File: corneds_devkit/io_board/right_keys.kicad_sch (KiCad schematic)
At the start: 42 parts, among them SW14 SW_Push, SW16 SW_Push, SW18 SW_Push, SW25 SW_Push, SW26 SW_Push, SW27 SW_Push, SW28 SW_Push, SW29 SW_Push, SW30 SW_Push, SW31 SW_Push, SW32 SW_Push, SW33 SW_Push, SW34 SW_Push, SW35 SW_Push, SW36 SW_Push, SW37 SW_Push, SW38 SW_Push, SW39 SW_Push, SW40 SW_Push, SW41 SW_Push, SW42 SW_Push

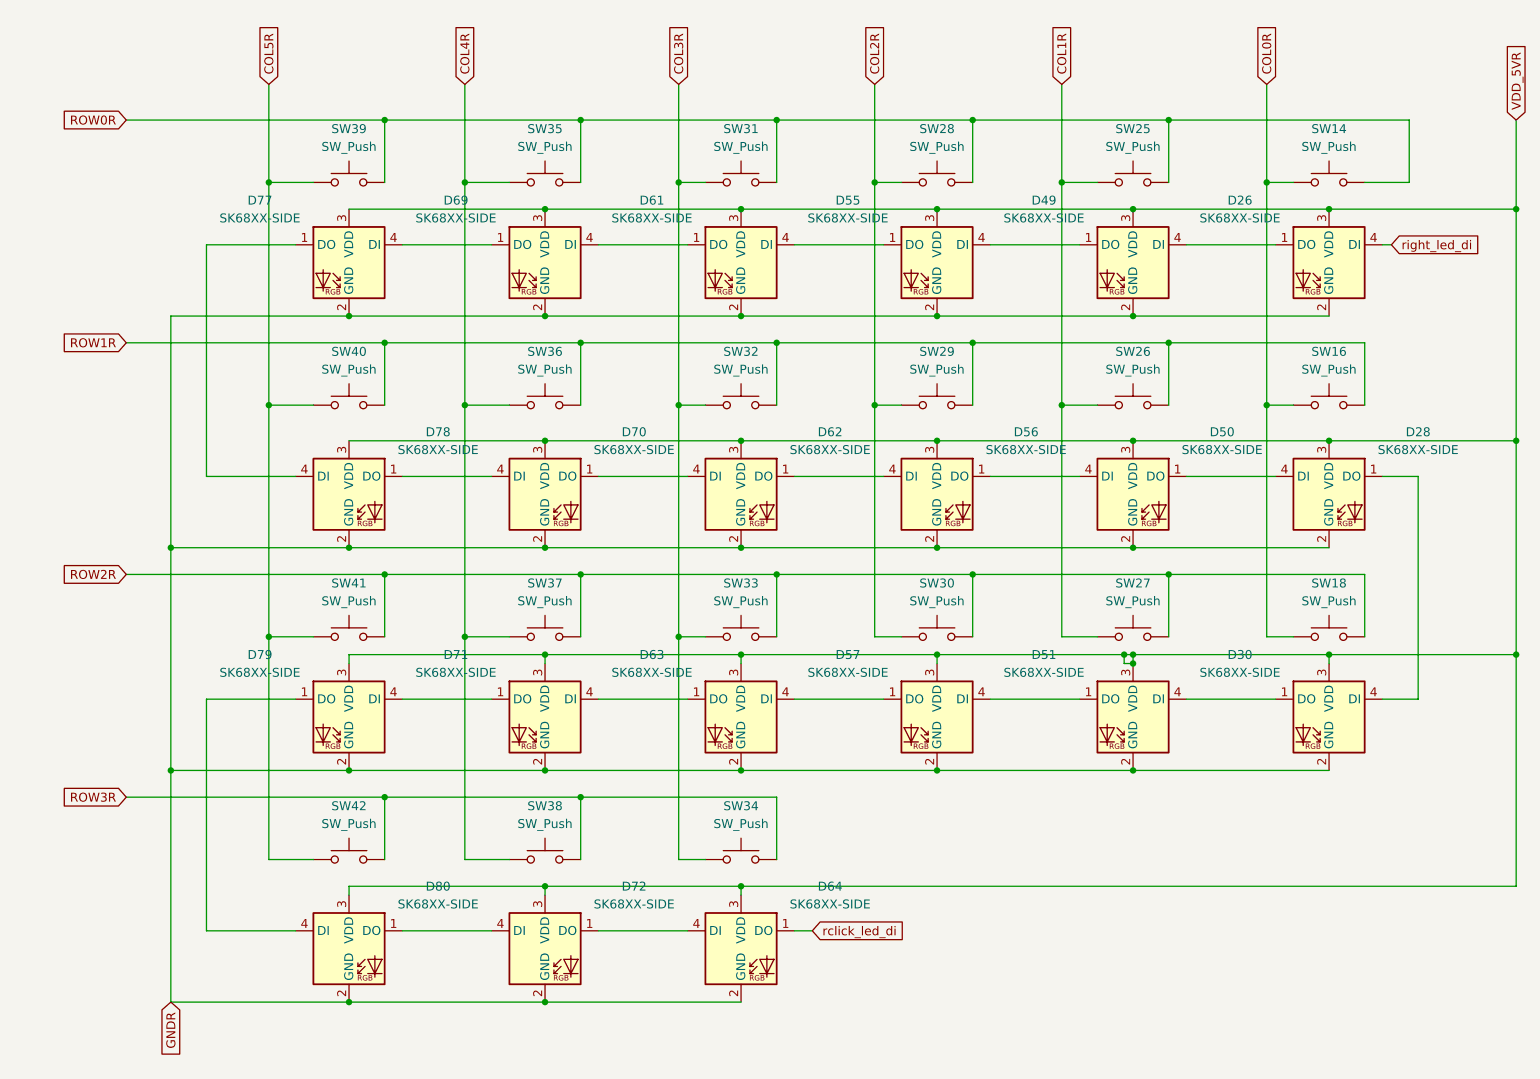
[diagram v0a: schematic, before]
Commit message: finished io board
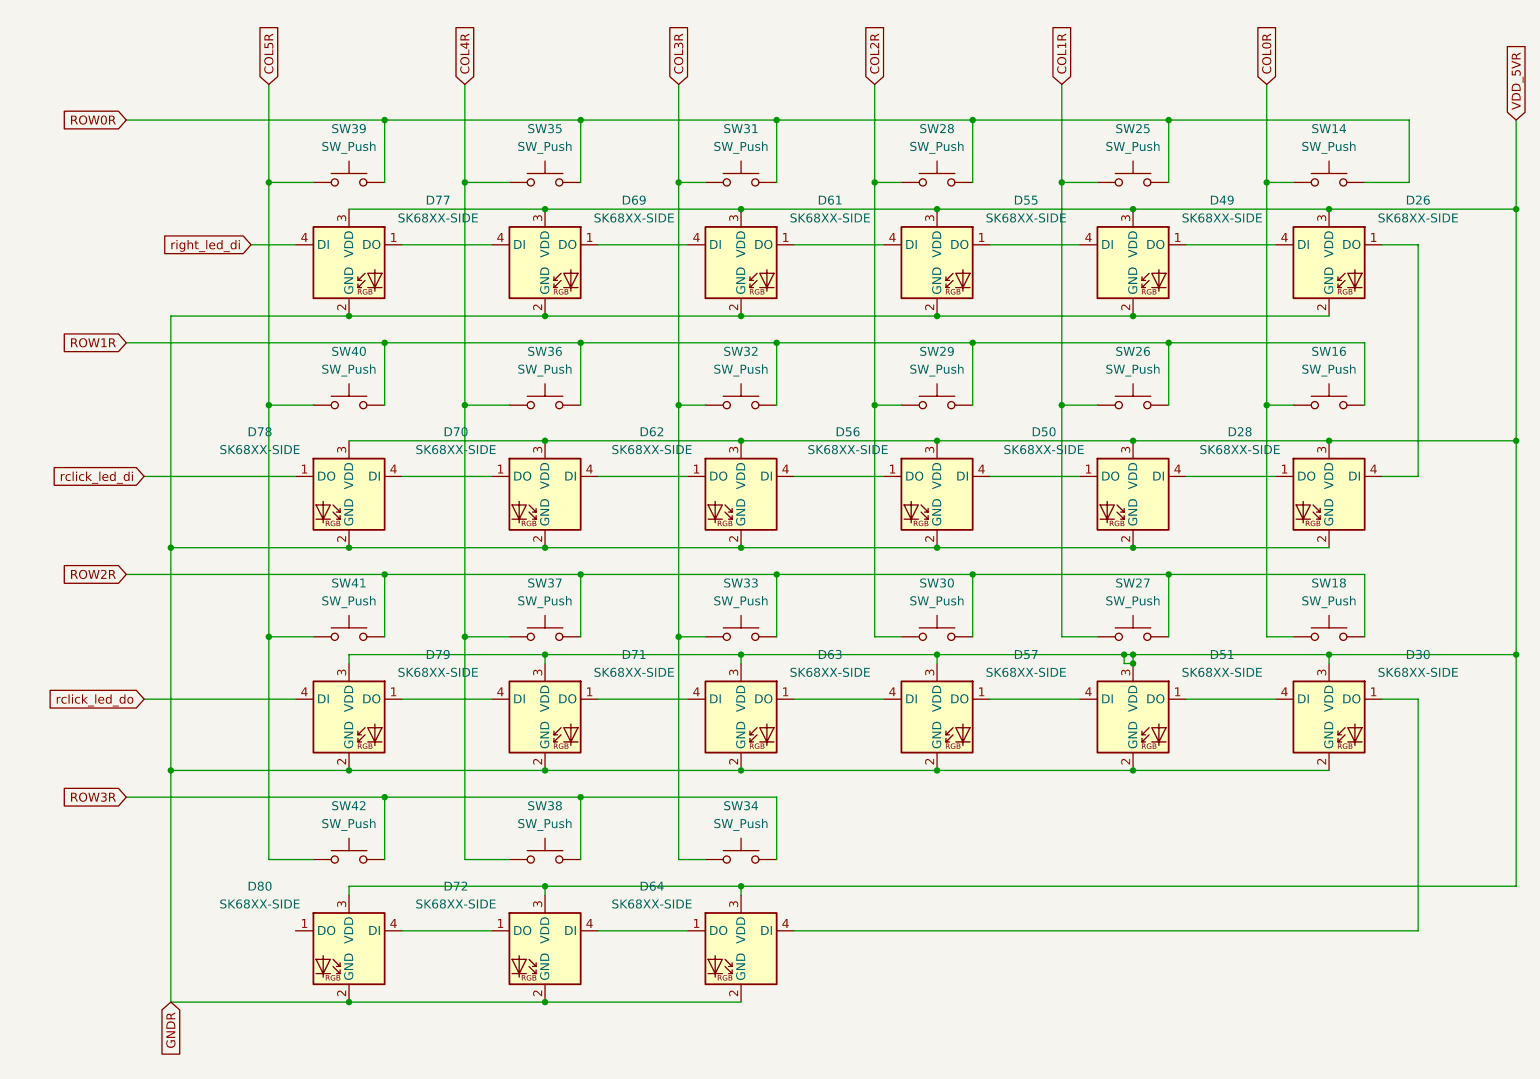
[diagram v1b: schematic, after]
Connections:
- net rclick_led_di: now also D78.1 (DO); no longer D64.1 (DO)
- net right_led_di: now also D77.4 (DI); no longer D26.4 (DI)
- net at D79.1 (DO): now also D71.4 (DI); no longer D80.4 (DI)
- net at D71.1 (DO): now also D63.4 (DI); no longer D79.4 (DI)
- net at D72.1 (DO): now also D80.4 (DI); no longer D64.4 (DI)
- net at D72.4 (DI): now also D64.1 (DO); no longer D80.1 (DO)
- net at D50.1 (DO): now also D56.4 (DI); no longer D28.4 (DI)
- net at D50.4 (DI): now also D28.1 (DO); no longer D56.1 (DO)
- net at D30.4 (DI): now also D51.1 (DO); no longer D28.1 (DO)
- net at D63.1 (DO): now also D57.4 (DI); no longer D71.4 (DI)
- net at D57.1 (DO): now also D51.4 (DI); no longer D63.4 (DI)
- net at D70.4 (DI): now also D62.1 (DO); no longer D78.1 (DO)
- net at D78.4 (DI): now also D70.1 (DO); no longer D77.1 (DO)
- net at D61.1 (DO): now also D55.4 (DI); no longer D69.4 (DI)
- net at D61.4 (DI): now also D69.1 (DO); no longer D55.1 (DO)
- net at D49.1 (DO): now also D26.4 (DI); no longer D55.4 (DI)
- net at D26.1 (DO): now also D28.4 (DI); no longer D49.4 (DI)
- net at D30.1 (DO): now also D64.4 (DI); no longer D51.4 (DI)
- net at D62.4 (DI): now also D56.1 (DO); no longer D70.1 (DO)
- new net: D69.4 (DI), D77.1 (DO)
- new net: D49.4 (DI), D55.1 (DO)
- new net rclick_led_do: D79.4 (DI)
